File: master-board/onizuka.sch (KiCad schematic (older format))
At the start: 30 parts, among them IC1 FT232RQ, IC2 ADCMP371, P1 USB_OTG, P2 FTDI, Q1 Q_PMOS_GSD, SW1 SPDT, U1 MIC5353-3.3YMT

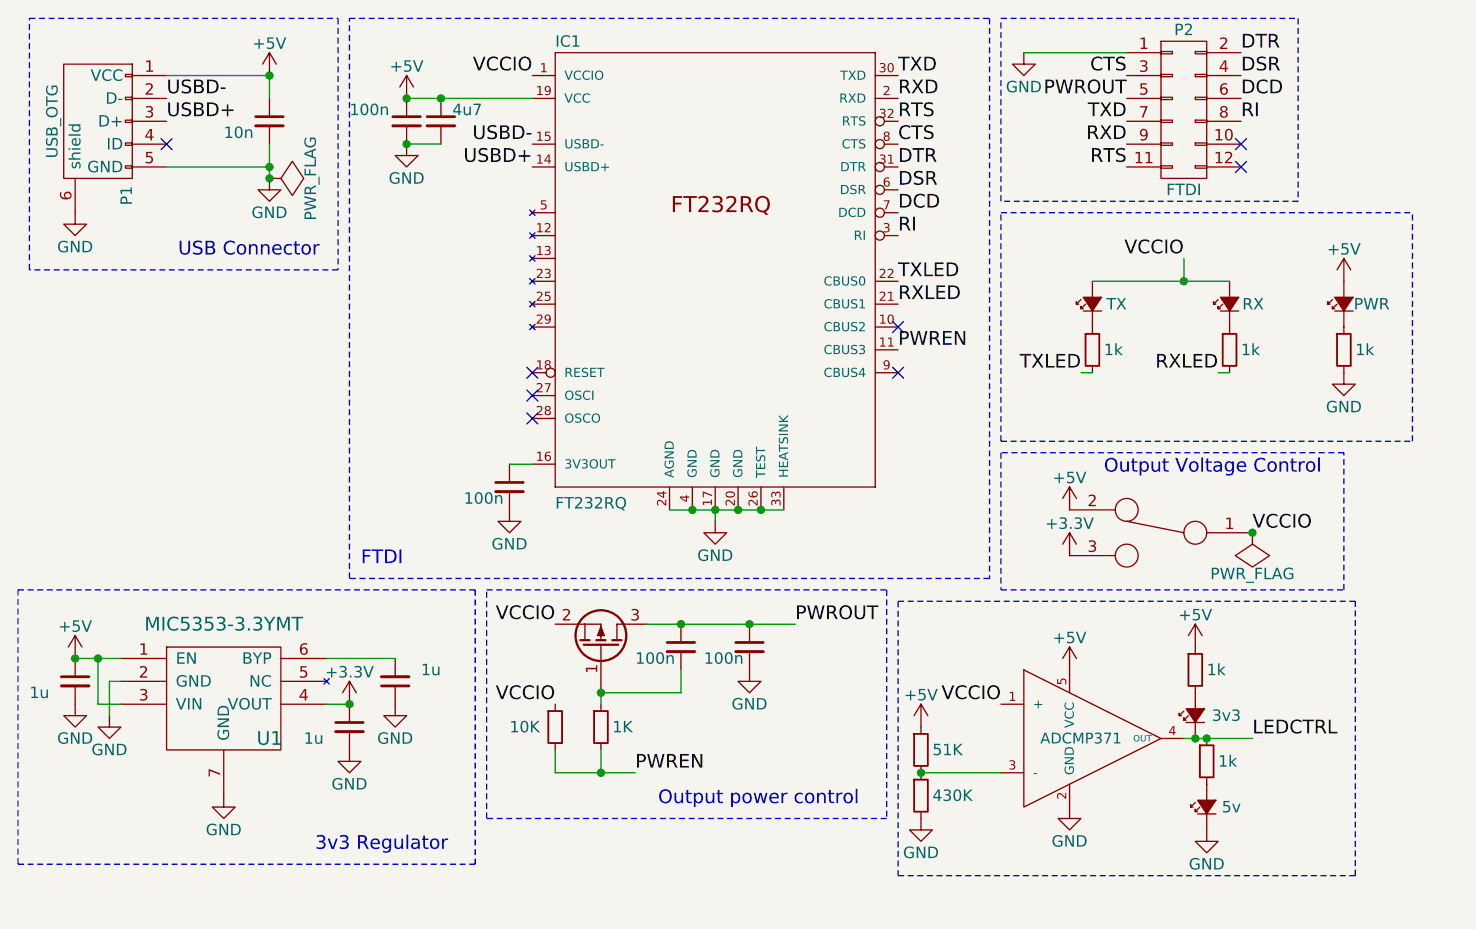
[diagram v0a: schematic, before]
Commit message: Many faffing, new ESP stuff.
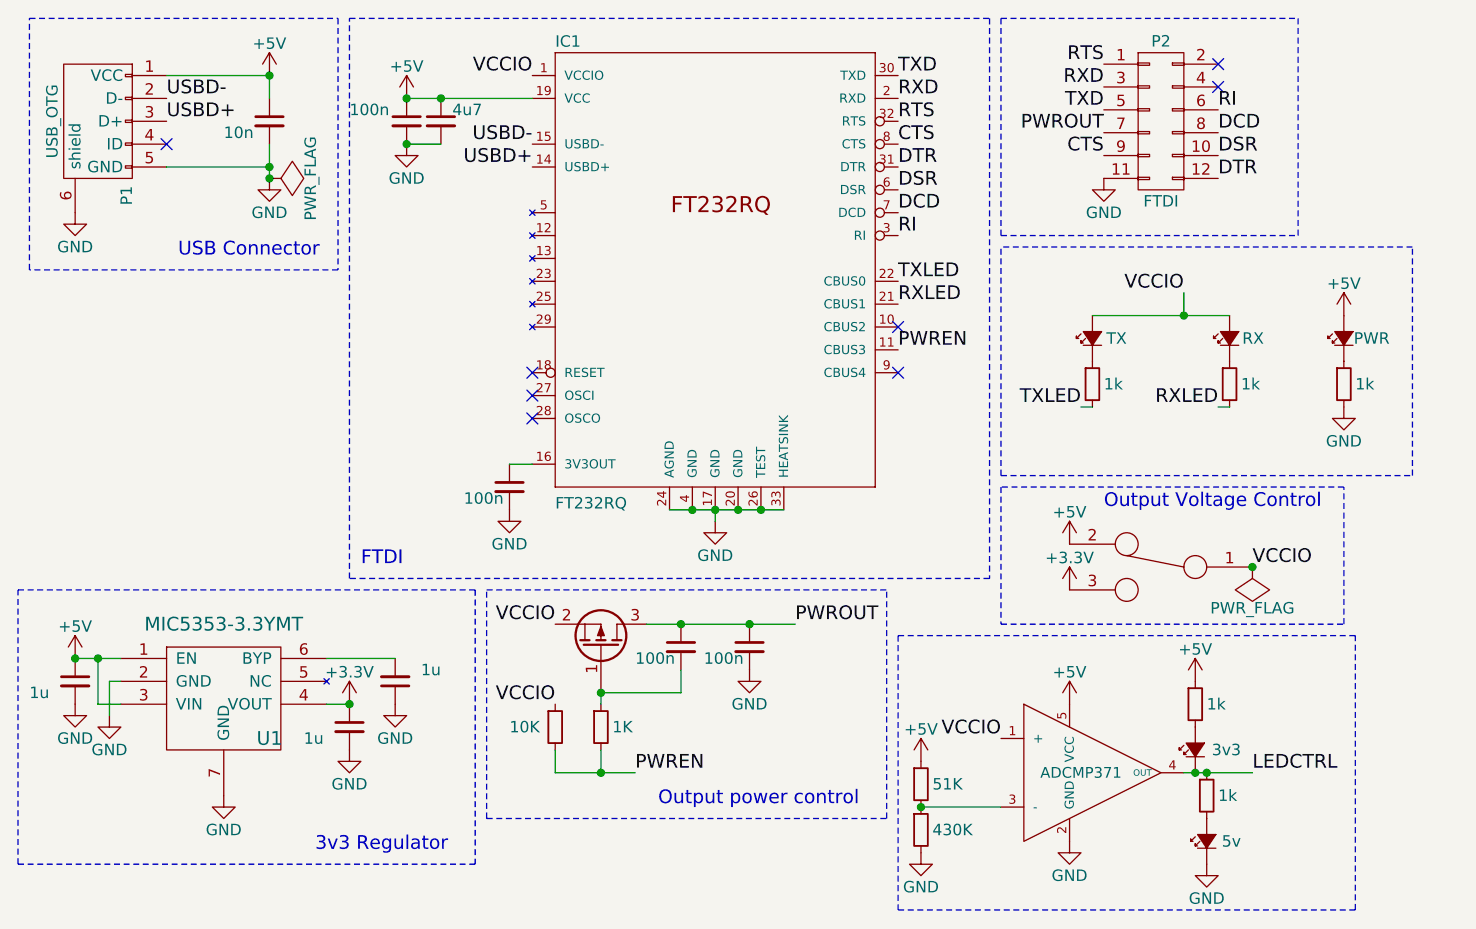
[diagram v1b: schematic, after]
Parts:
- P2: footprint Pin_Headers:Pin_Header_Angled_2x06 -> Socket_Strips:Socket_Strip_Angled_2x06
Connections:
- net CTS: now also P2.9 (P9); no longer P2.3 (P3)
- net DCD: now also P2.8 (P8); no longer P2.6 (P6)
- net DSR: now also P2.10 (P10); no longer P2.4 (P4)
- net DTR: now also P2.12 (P12); no longer P2.2 (P2)
- net GND: now also P2.11 (P11); no longer P2.1 (P1)
- net PWROUT: now also P2.7 (P7); no longer P2.5 (P5)
- net RI: now also P2.6 (P6); no longer P2.8 (P8)
- net RTS: now also P2.1 (P1); no longer P2.11 (P11)
- net RXD: now also P2.3 (P3); no longer P2.9 (P9)
- net TXD: now also P2.5 (P5); no longer P2.7 (P7)
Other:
- moved on the sheet: P2

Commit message: Various shuffling, adding farnell part numbers.
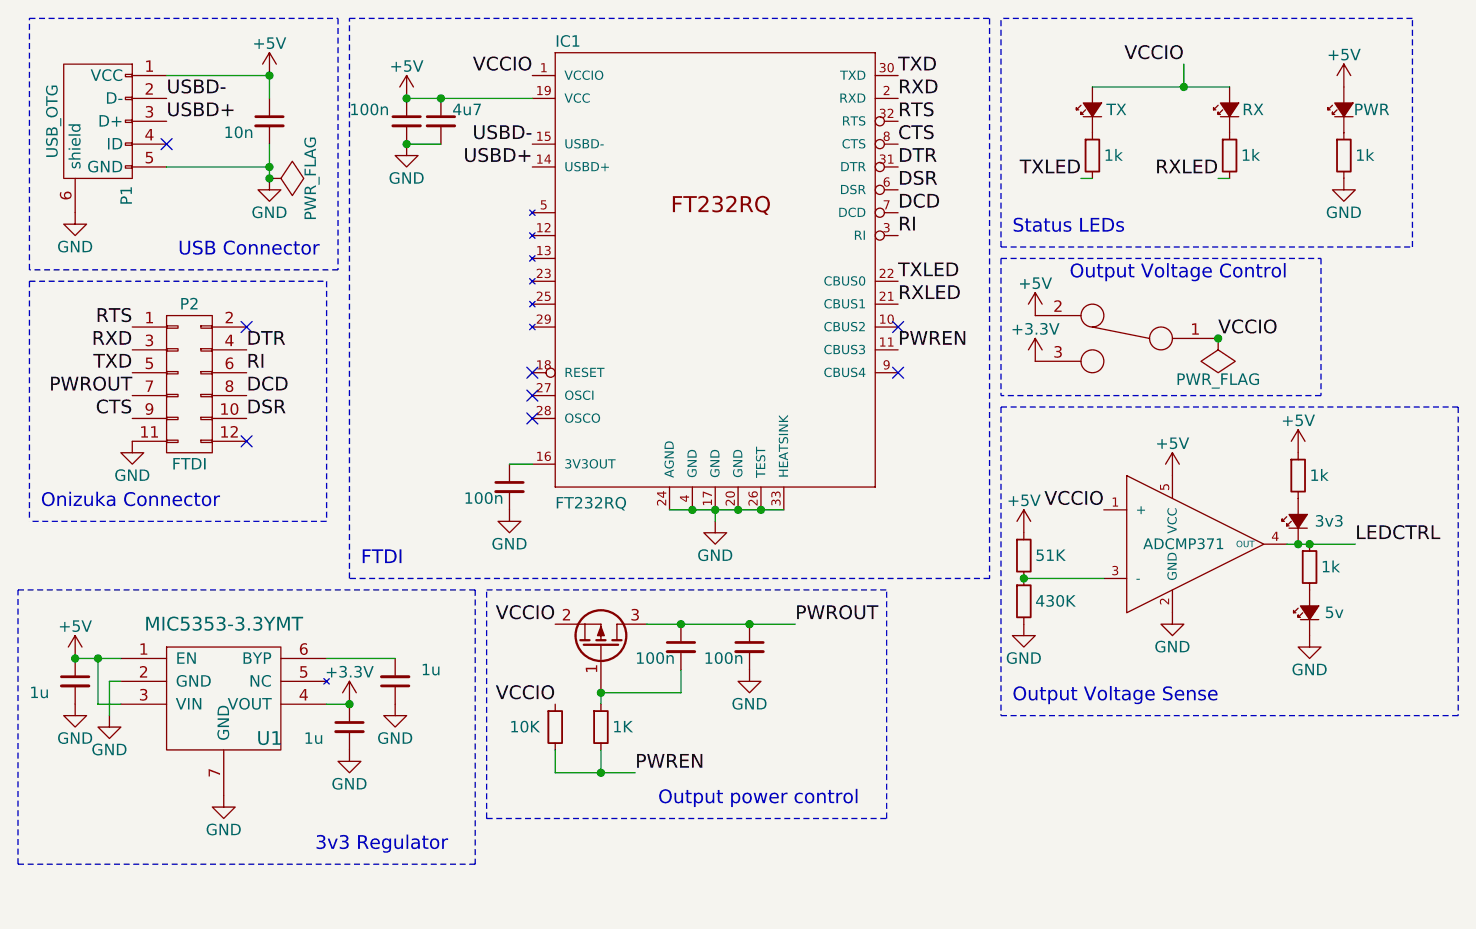
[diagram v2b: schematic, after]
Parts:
- IC1: Farnell (none) -> 1146033
- P2: Farnell (none) -> 1668355
- R1, R2, R3, R4, R7, R8: Farnell (none) -> 2498165
- SW1: Farnell (none) -> 2134452
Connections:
- net DTR: now also P2.4 (P4); no longer P2.12 (P12)
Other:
- note added: "Onizuka Connector"
- note added: "Output Voltage Sense"
- note added: "Status LEDs"
- moved on the sheet: P2
